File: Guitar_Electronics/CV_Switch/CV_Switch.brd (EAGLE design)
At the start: 39 x 33 mm, 7 parts

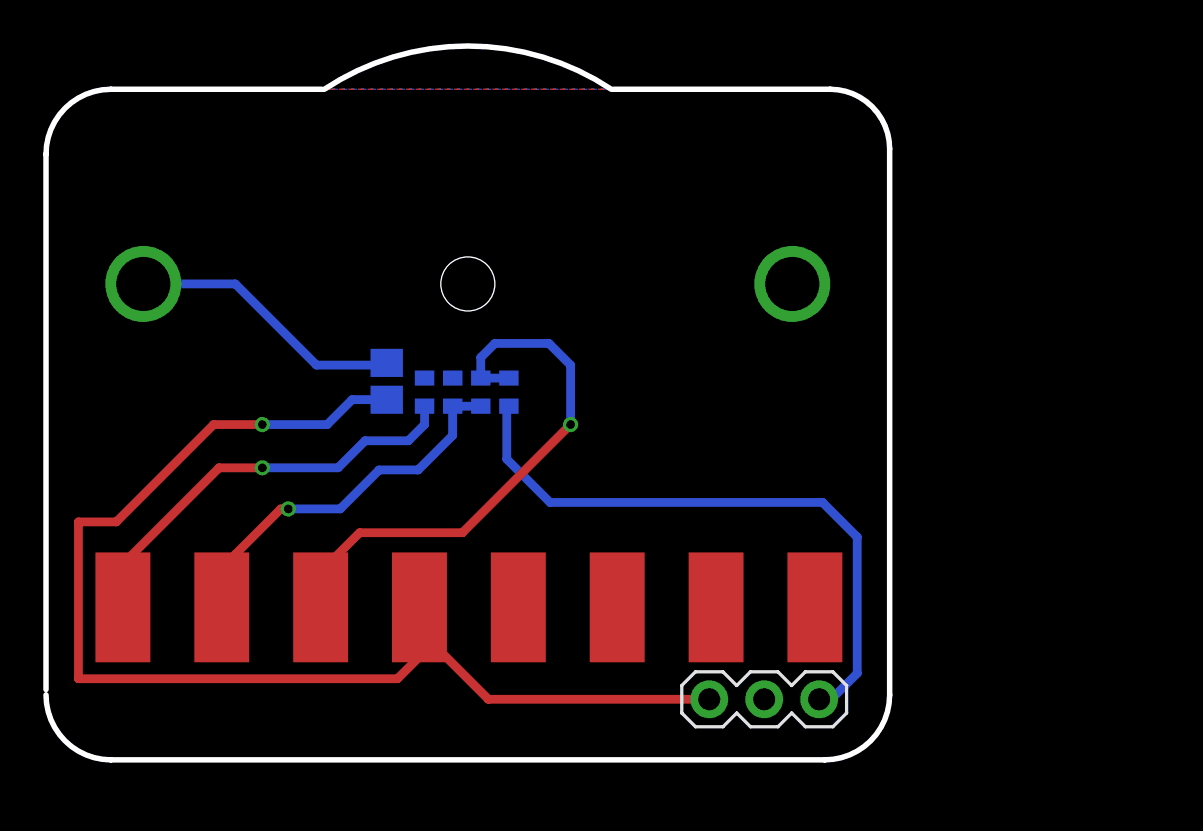
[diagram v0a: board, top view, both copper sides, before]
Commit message: Licenses
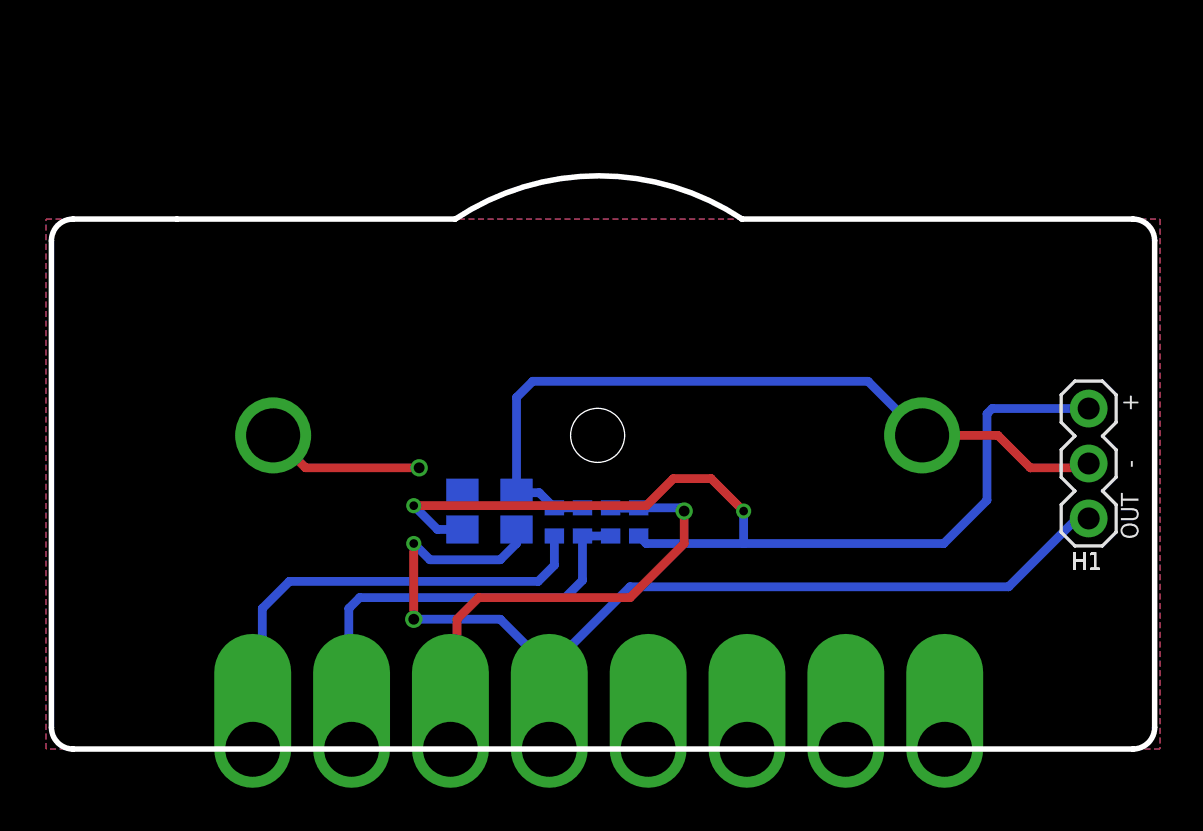
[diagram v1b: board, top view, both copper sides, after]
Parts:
- added C2: 10uF, resistor:C0805
- C1: value 0.1uF -> 10uF
- U$1: value 5WAY_SW_1_ -> 5WAY_SW_1; device CYCFI_switch:5WAY_SW -> CYCFI_switch:5WAY_SW_CASTELLATED
- moved H1 18.5 mm to (48.2, 13.7), turned to 90 degrees
- moved U$1 8.89 mm to (25.6, 0.49)
- moved C1 8.49 mm to (21.8, 11.5)
- moved R1 8.49 mm to (27.4, 11.0)
- moved R2 8.49 mm to (26.1, 11.0)
- moved R3 8.49 mm to (24.8, 11.0)
- moved R4 8.49 mm to (23.5, 11.0)
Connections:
- net GND: now also C2.2
- net N$1: now also C2.1
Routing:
- net GND: track 12.8 -> 43.8 mm, vias 2 -> 3
- net N$1: track 28.8 -> 46.5 mm, vias 0 -> 2
- net OUT: track 56.7 -> 48.5 mm, vias 1 -> 2
- net N$6: track 17.7 -> 21.3 mm, vias 1 -> 0
- net N$3: track 19.5 -> 22.4 mm, vias 1 -> 0
- net N$2: track 25.9 -> 24.4 mm
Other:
- board size 39 x 33 mm -> 51 x 26.5 mm
- board text added: "v0.97"
- board text removed: "v0.92"
